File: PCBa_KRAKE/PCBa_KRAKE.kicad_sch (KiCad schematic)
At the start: 51 parts, among them J101 Barrel_Jack_Switch_SMT, J102 0.100_2Pin, J103 0.100_2Pin, J105 S04B-XASK-1(LF)(SN)Rev2, U101 LM7805_TO220, U102 PI_ATMEGA328P-AU-InOrder, U999 ESP32-WROOM-32D

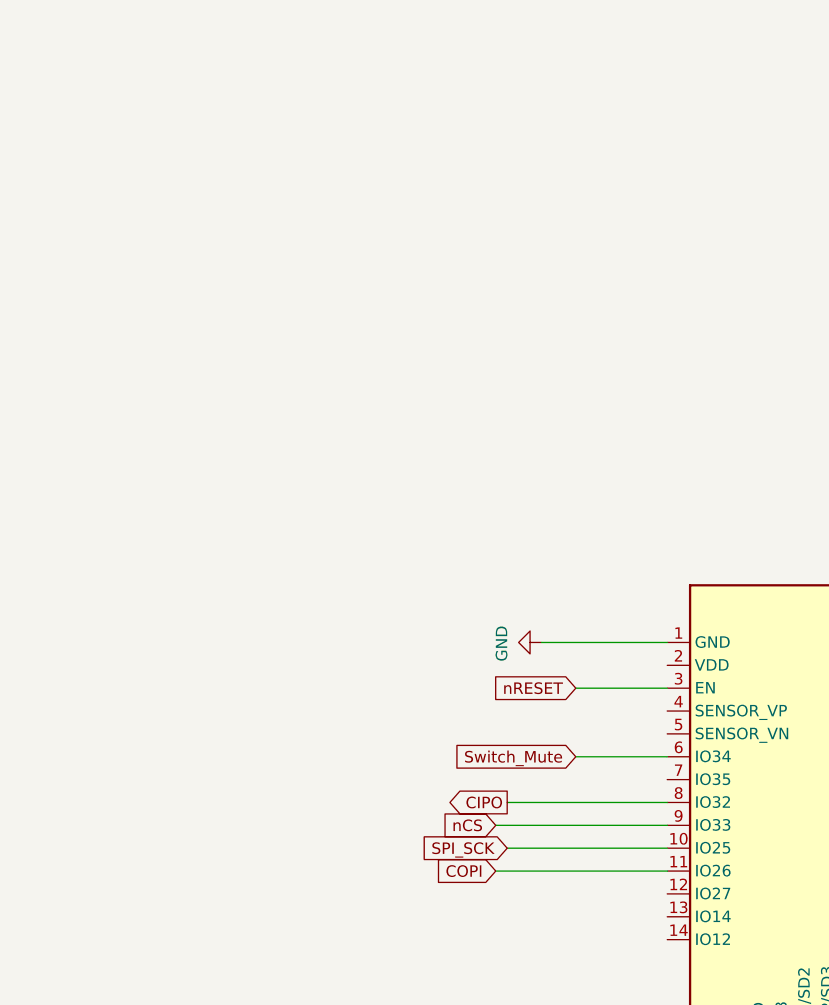
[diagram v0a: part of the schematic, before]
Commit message: PCBa_KRAKE.kicad_sch adding 3v3 voltage regulator.
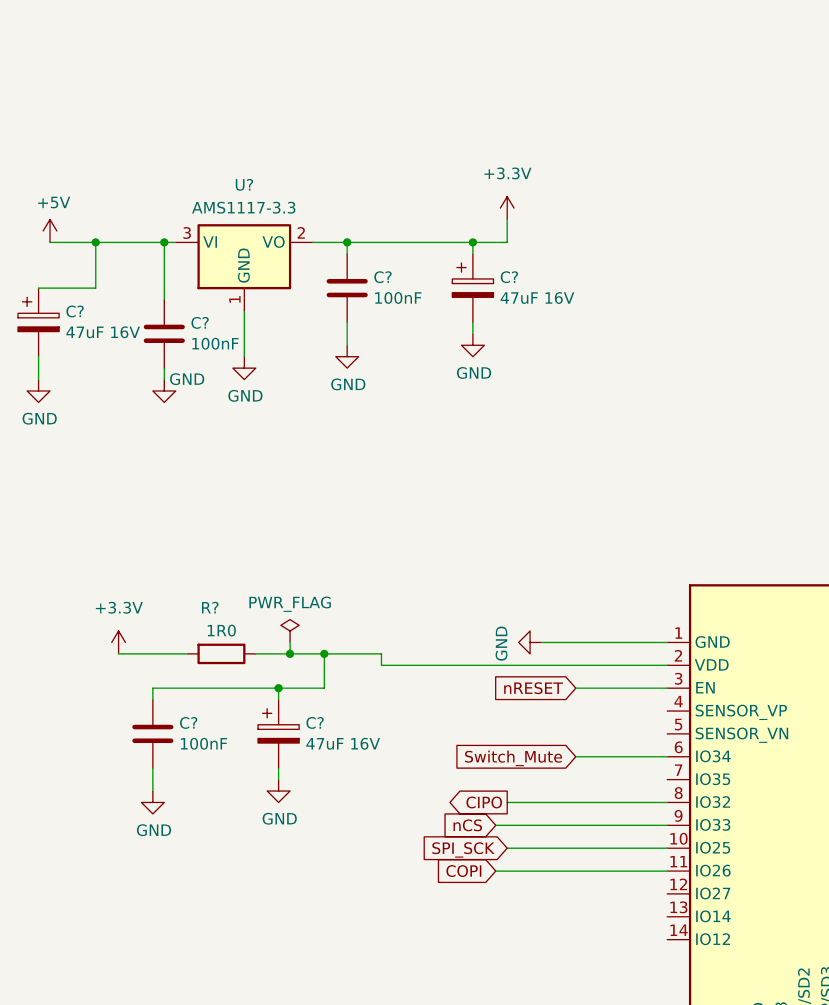
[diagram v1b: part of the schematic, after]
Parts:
- added C? (x3): 47uF 16V, Capacitor_SMD:CP_Elec_5x5.4, symbol Device:C_Polarized
- added C? (x3): 100nF, Capacitor_SMD:C_0603_1608Metric_Pad1.08x0.95mm_HandSolder, symbol Device:C
- added R?: 1R0, Resistor_SMD:R_0603_1608Metric_Pad0.98x0.95mm_HandSolder, symbol Device:R
- added U?: AMS1117-3.3, Package_TO_SOT_SMD:SOT-223-3_TabPin2, symbol Regulator_Linear:AMS1117-3.3
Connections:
- net +5V: now also C?.1, C?.1, U?.3 (VI)
- net GND: now also C?.2, C?.2, C?.2, C?.2, C?.2, C?.2, U?.1 (GND)
- net at U999.2 (VDD): now also C?.1, C?.1, R?.1
- new net +3.3V: C?.1, C?.1, R?.2, U?.2 (VO)
